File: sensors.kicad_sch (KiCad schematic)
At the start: 5 parts, among them U2 LIS2MDL

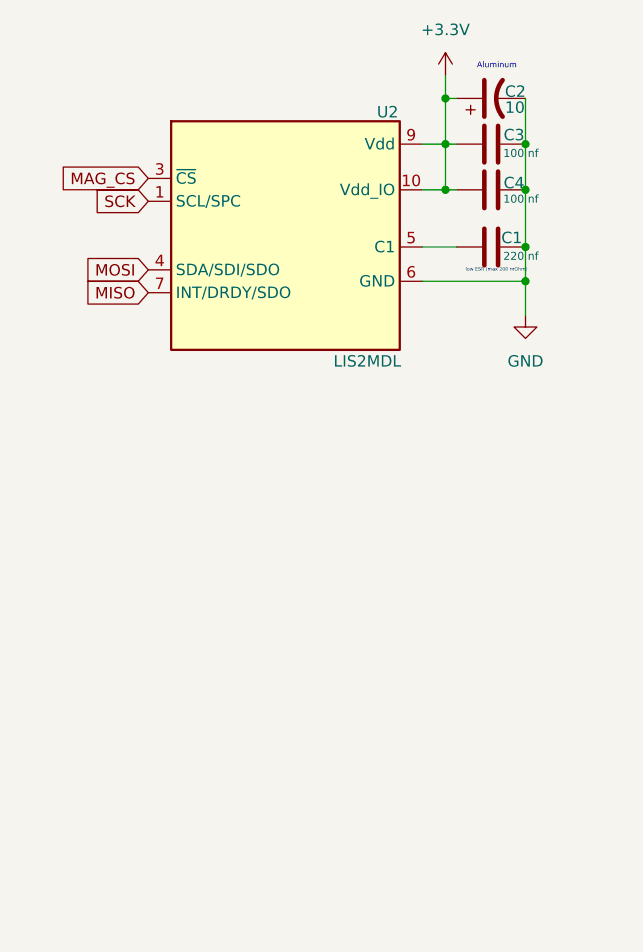
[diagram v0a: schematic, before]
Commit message: Add files via upload
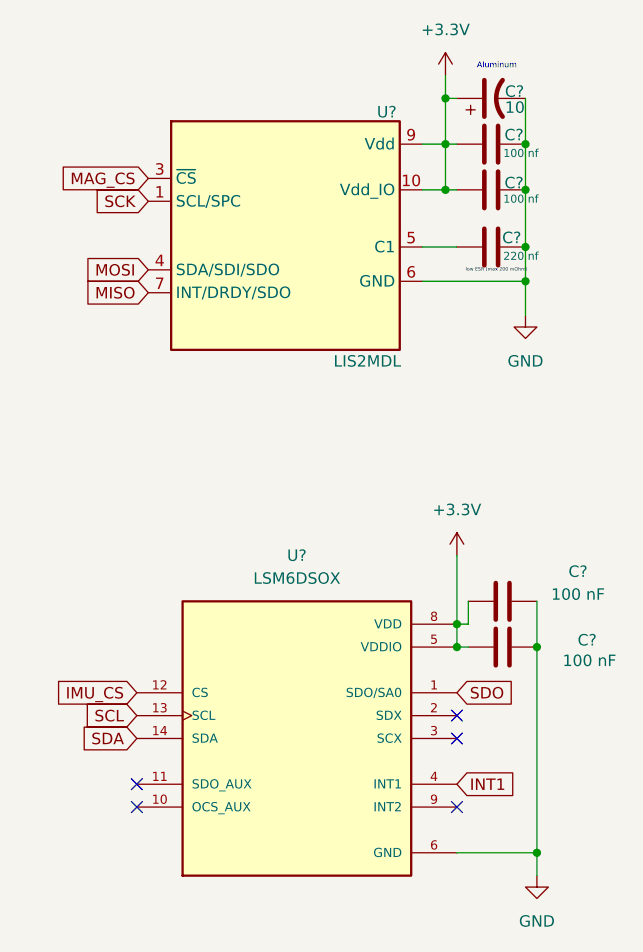
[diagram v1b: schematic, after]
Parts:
- added C? (x2): 100 nF, symbol Device:C
- added U?: LSM6DSOX, symbol imu:LSM6DSOX
- renumbered C3 to C?, C2 to C?, C1 to C?, C4 to C?, U2 to U?
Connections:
- net +3.3V: now also C?.1, C?.1, U?.5 (VDDIO), U?.8 (VDD)
- net GND: now also C?.2, C?.2, U?.6 (GND), U?.7 (GND)
- new net IMU_CS: U?.12 (CS)
- new net INT1: U?.4 (INT1)
- new net SCL: U?.13 (SCL)
- new net SDA: U?.14 (SDA)
- new net SDO: U?.1 (SDO/SA0)
- no-connect marks 0 -> 5

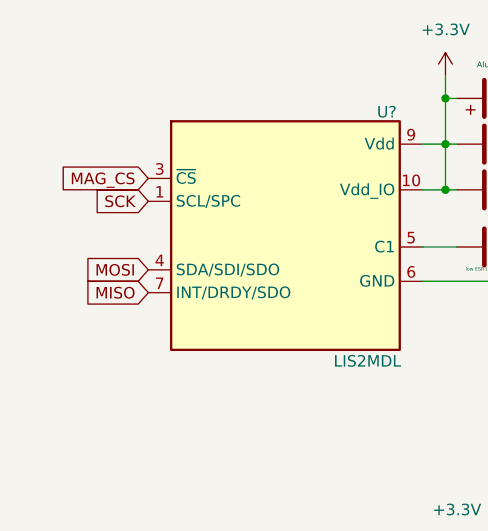
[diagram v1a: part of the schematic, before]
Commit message: Just updated some labels in the schematic.
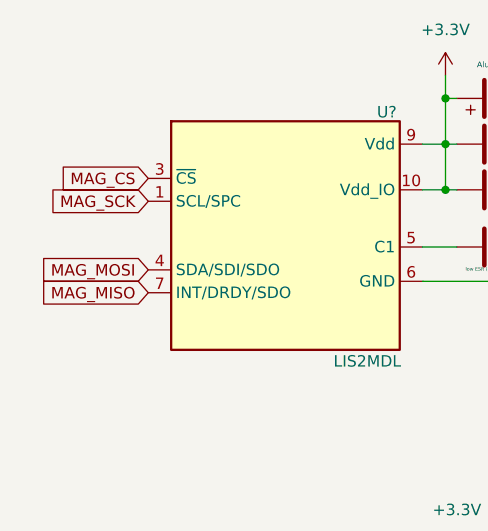
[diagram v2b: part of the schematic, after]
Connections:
- net MISO renamed MAG_MISO
- net MOSI renamed MAG_MOSI
- net SCK renamed MAG_SCK
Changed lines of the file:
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@@
 		)
 	)
-	(global_label "MOSI"
+	(global_label "MAG_MOSI"
 		(shape input)
 		(at 49.53 53.34 180)
@@
 		)
 		(property "Intersheetrefs" "${INTERSHEET_REFS}"
-			(at 41.9486 53.34 0)
+			(at 37.171 53.34 0)
 			(effects
 				(font
@@
 		)
 	)
-	(global_label "MISO"
+	(global_label "MAG_MISO"
 		(shape input)
 		(at 49.53 55.88 180)
@@
 		)
 		(property "Intersheetrefs" "${INTERSHEET_REFS}"
-			(at 41.9486 55.88 0)
+			(at 37.171 55.88 0)
 			(effects
 				(font
@@
 		)
 	)
-	(global_label "SCK"
+	(global_label "MAG_SCK"
 		(shape input)
 		(at 49.53 45.72 180)
@@
 		)
 		(property "Intersheetrefs" "${INTERSHEET_REFS}"
-			(at 42.7953 45.72 0)
+			(at 38.0177 45.72 0)
 			(effects
 				(font
@@
 		)
 		(instances
-			(project "flight-controller-basic (1)"
-				(path "/e04fbe87-dc7c-407c-abef-b71ed1bbe06a/bae430cb-0c9f-4691-9dd7-9716141b7e53"
+			(project "flight-controller-basic"
+				(path "/e04fbe87-dc7c-407c-abef-b71ed1bbe06a/15ccaa96-ad63-4a4d-bfcd-1e00695c7116"
 					(reference "C?")
 					(unit 1)
@@
 		)
 		(instances
-			(project "flight-controller-basic (1)"
-				(path "/e04fbe87-dc7c-407c-abef-b71ed1bbe06a/bae430cb-0c9f-4691-9dd7-9716141b7e53"
+			(project "flight-controller-basic"
+				(path "/e04fbe87-dc7c-407c-abef-b71ed1bbe06a/15ccaa96-ad63-4a4d-bfcd-1e00695c7116"
 					(reference "C?")
 					(unit 1)
@@
 		)
 		(instances
-			(project "flight-controller-basic (1)"
-				(path "/e04fbe87-dc7c-407c-abef-b71ed1bbe06a/bae430cb-0c9f-4691-9dd7-9716141b7e53"
+			(project "flight-controller-basic"
+				(path "/e04fbe87-dc7c-407c-abef-b71ed1bbe06a/15ccaa96-ad63-4a4d-bfcd-1e00695c7116"
 					(reference "#PWR?")
 					(unit 1)
@@
 		)
 		(instances
-			(project "flight-controller-basic (1)"
-				(path "/e04fbe87-dc7c-407c-abef-b71ed1bbe06a/bae430cb-0c9f-4691-9dd7-9716141b7e53"
+			(project "flight-controller-basic"
+				(path "/e04fbe87-dc7c-407c-abef-b71ed1bbe06a/15ccaa96-ad63-4a4d-bfcd-1e00695c7116"
 					(reference "C?")
 					(unit 1)
@@
 		)
 		(instances
-			(project "flight-controller-basic (1)"
-				(path "/e04fbe87-dc7c-407c-abef-b71ed1bbe06a/bae430cb-0c9f-4691-9dd7-9716141b7e53"
+			(project "flight-controller-basic"
+				(path "/e04fbe87-dc7c-407c-abef-b71ed1bbe06a/15ccaa96-ad63-4a4d-bfcd-1e00695c7116"
 					(reference "#PWR?")
 					(unit 1)
@@
 		)
 		(instances
-			(project "flight-controller-basic (1)"
-				(path "/e04fbe87-dc7c-407c-abef-b71ed1bbe06a/bae430cb-0c9f-4691-9dd7-9716141b7e53"
+			(project "flight-controller-basic"
+				(path "/e04fbe87-dc7c-407c-abef-b71ed1bbe06a/15ccaa96-ad63-4a4d-bfcd-1e00695c7116"
 					(reference "C?")
 					(unit 1)
@@
 		)
 		(instances
-			(project "flight-controller-basic (1)"
-				(path "/e04fbe87-dc7c-407c-abef-b71ed1bbe06a/bae430cb-0c9f-4691-9dd7-9716141b7e53"
+			(project "flight-controller-basic"
+				(path "/e04fbe87-dc7c-407c-abef-b71ed1bbe06a/15ccaa96-ad63-4a4d-bfcd-1e00695c7116"
 					(reference "#PWR?")
 					(unit 1)
@@
 		)
 		(instances
-			(project "flight-controller-basic (1)"
-				(path "/e04fbe87-dc7c-407c-abef-b71ed1bbe06a/bae430cb-0c9f-4691-9dd7-9716141b7e53"
+			(project "flight-controller-basic"
+				(path "/e04fbe87-dc7c-407c-abef-b71ed1bbe06a/15ccaa96-ad63-4a4d-bfcd-1e00695c7116"
 					(reference "C?")
 					(unit 1)
@@
 		)
 		(instances
-			(project "flight-controller-basic (1)"
-				(path "/e04fbe87-dc7c-407c-abef-b71ed1bbe06a/bae430cb-0c9f-4691-9dd7-9716141b7e53"
+			(project "flight-controller-basic"
+				(path "/e04fbe87-dc7c-407c-abef-b71ed1bbe06a/15ccaa96-ad63-4a4d-bfcd-1e00695c7116"
 					(reference "U?")
 					(unit 1)
@@
 		)
 		(instances
-			(project "flight-controller-basic (1)"
-				(path "/e04fbe87-dc7c-407c-abef-b71ed1bbe06a/bae430cb-0c9f-4691-9dd7-9716141b7e53"
+			(project "flight-controller-basic"
+				(path "/e04fbe87-dc7c-407c-abef-b71ed1bbe06a/15ccaa96-ad63-4a4d-bfcd-1e00695c7116"
 					(reference "U?")
 					(unit 1)
@@
 		)
 		(instances
-			(project "flight-controller-basic (1)"
-				(path "/e04fbe87-dc7c-407c-abef-b71ed1bbe06a/bae430cb-0c9f-4691-9dd7-9716141b7e53"
+			(project "flight-controller-basic"
+				(path "/e04fbe87-dc7c-407c-abef-b71ed1bbe06a/15ccaa96-ad63-4a4d-bfcd-1e00695c7116"
 					(reference "C?")
 					(unit 1)
@@
 		)
 		(instances
-			(project "flight-controller-basic (1)"
-				(path "/e04fbe87-dc7c-407c-abef-b71ed1bbe06a/bae430cb-0c9f-4691-9dd7-9716141b7e53"
+			(project "flight-controller-basic"
+				(path "/e04fbe87-dc7c-407c-abef-b71ed1bbe06a/15ccaa96-ad63-4a4d-bfcd-1e00695c7116"
 					(reference "#PWR?")
 					(unit 1)
